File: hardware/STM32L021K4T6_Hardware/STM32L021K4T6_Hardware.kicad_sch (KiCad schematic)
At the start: 1 part, among them U1 STM32L021K4Tx

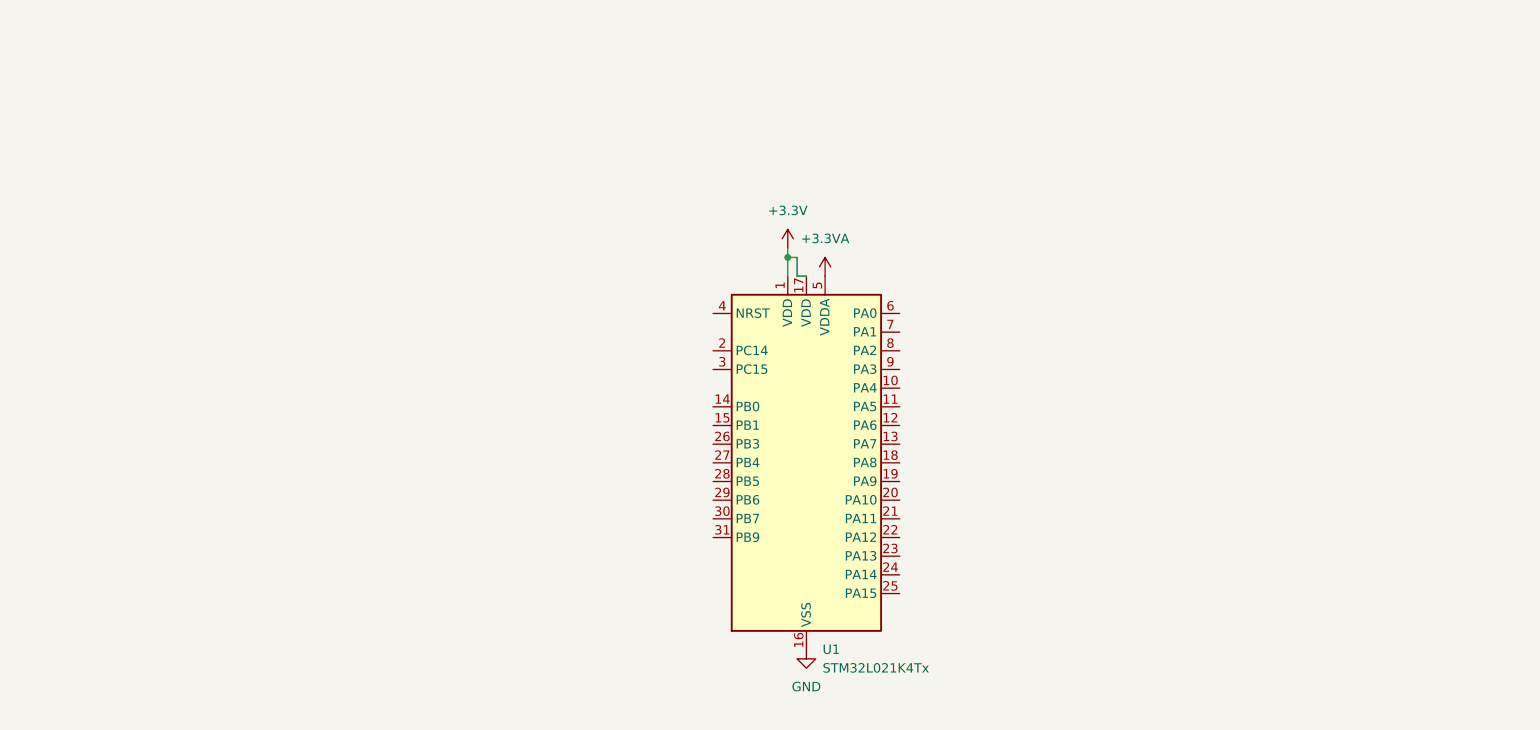
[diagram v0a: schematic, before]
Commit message: schematic and footprints
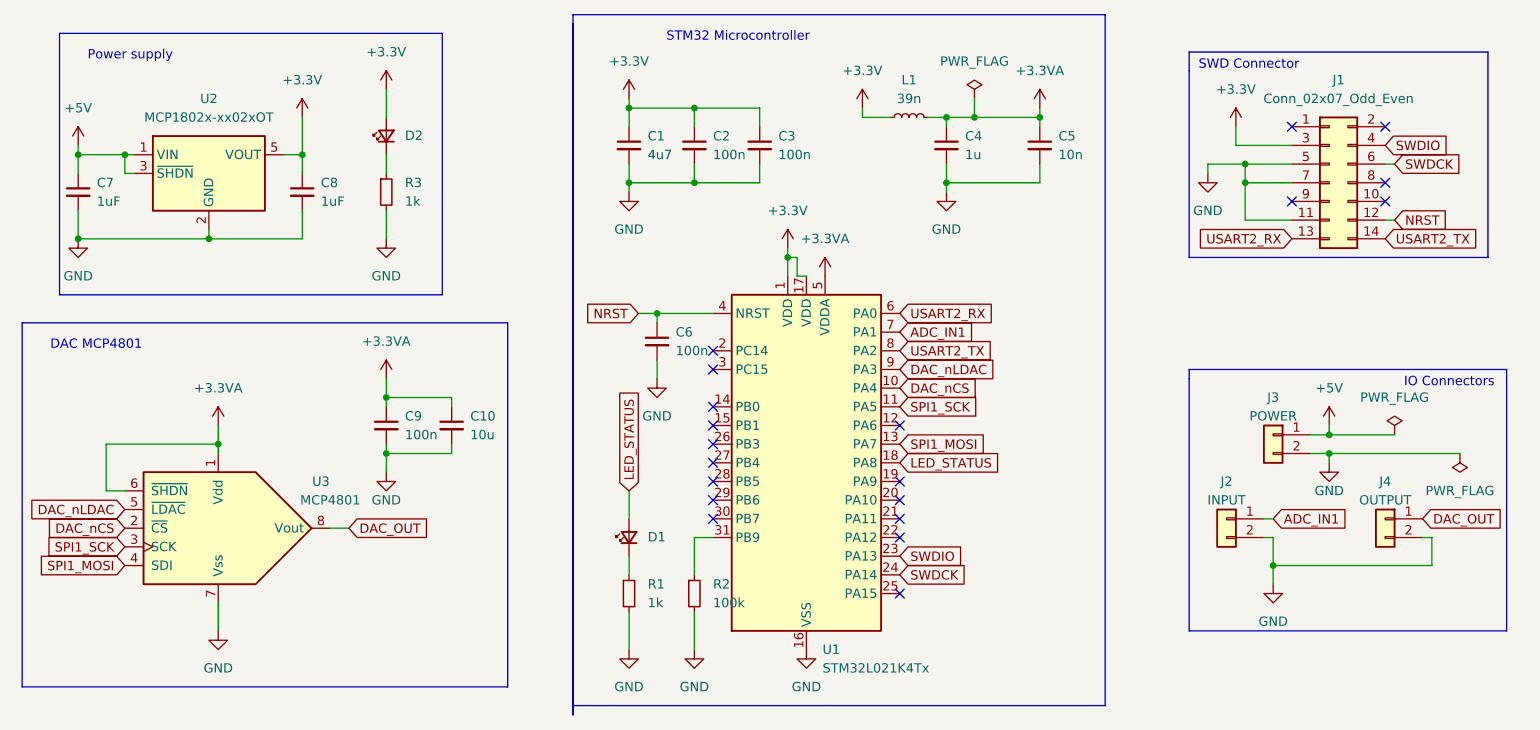
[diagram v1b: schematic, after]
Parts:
- added C1: 4u7, Capacitor_SMD:C_0805_2012Metric_Pad1.18x1.45mm_HandSolder, symbol Device:C_Small
- added C10: 10u, Capacitor_SMD:C_0805_2012Metric, symbol Device:C_Small
- added C2, C3, C6, C9: 100n, Capacitor_SMD:C_0805_2012Metric_Pad1.18x1.45mm_HandSolder, symbol Device:C_Small
- added C4: 1u, Capacitor_SMD:C_0805_2012Metric_Pad1.18x1.45mm_HandSolder, symbol Device:C_Small
- added C5: 10n, Capacitor_SMD:C_0805_2012Metric_Pad1.18x1.45mm_HandSolder, symbol Device:C_Small
- added C7, C8: 1uF, Capacitor_SMD:C_0805_2012Metric, symbol Device:C_Small
- added D1, D2: ~, LED_SMD:LED_0603_1608Metric_Pad1.05x0.95mm_HandSolder, symbol Device:LED_Small
- added J1: Conn_02x07_Odd_Even, Connector_PinHeader_1.27mm:PinHeader_2x07_P1.27mm_Vertical_SMD, symbol Connector_Generic:Conn_02x07_Odd_Even
- added J2: INPUT, Connector_JST:JST_XH_B2B-XH-A_1x02_P2.50mm_Vertical, symbol Connector_Generic:Conn_01x02
- added J3: POWER, Connector_JST:JST_XH_B2B-XH-A_1x02_P2.50mm_Vertical, symbol Connector_Generic:Conn_01x02
- added J4: OUTPUT, Connector_JST:JST_XH_B2B-XH-A_1x02_P2.50mm_Vertical, symbol Connector_Generic:Conn_01x02
- added L1: 39n, Inductor_SMD:L_0805_2012Metric_Pad1.05x1.20mm_HandSolder, symbol Device:L_Small
- added R1, R3: 1k, Resistor_SMD:R_0805_2012Metric_Pad1.20x1.40mm_HandSolder, symbol Device:R_Small
- added R2: 100k, Resistor_SMD:R_0805_2012Metric_Pad1.20x1.40mm_HandSolder, symbol Device:R_Small
- added U2: MCP1802x-xx02xOT, Package_TO_SOT_SMD:SOT-23-5, symbol Regulator_Linear:MCP1802x-xx02xOT
- added U3: MCP4801, Package_SO:SOIC-8_3.9x4.9mm_P1.27mm, symbol Analog_DAC:MCP4801
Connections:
- net +3.3V: now also C1.1, C2.1, C3.1, C8.1, D2.2 (A), J1.3 (Pin_3), L1.1, U2.5 (VOUT)
- net +3.3VA: now also C10.1, C4.1, C5.1, C9.1, L1.2, U3.1 (Vdd), U3.6 (~{SHDN})
- net GND: now also C1.2, C10.2, C2.2, C3.2, C4.2, C5.2, C6.2, C7.2, C8.2, C9.2, J1.11 (Pin_11), J1.5 (Pin_5), J1.7 (Pin_7), J2.2 (Pin_2), J3.2 (Pin_2), J4.2 (Pin_2), R1.2, R2.2, R3.2, U2.2 (GND), U3.7 (Vss)
- net DAC_nCS: now reaches U1.10 (PA4)
- net DAC_nCS: now also U3.2 (~{CS})
- net SPI1_SCK: now reaches U1.11 (PA5)
- net SPI1_SCK: now also U3.3 (SCK)
- net SPI1_MOSI: now reaches U1.13 (PA7)
- net SPI1_MOSI: now also U3.4 (SDI)
- net LED_STATUS: now reaches U1.18 (PA8)
- net LED_STATUS: now also D1.2 (A)
- net SWDIO: now reaches U1.23 (PA13)
- net SWDIO: now also J1.4 (Pin_4)
- net SWDCK: now reaches U1.24 (PA14)
- net SWDCK: now also J1.6 (Pin_6)
- net at U1.31 (PB9): now also R2.1
- net NRST: now reaches U1.4 (NRST)
- net NRST: now also C6.1, J1.12 (Pin_12)
- net USART2_RX: now reaches U1.6 (PA0)
- net USART2_RX: now also J1.13 (Pin_13)
- net ADC_IN1: now reaches U1.7 (PA1)
- net ADC_IN1: now also J2.1 (Pin_1)
- net USART2_TX: now reaches U1.8 (PA2)
- net USART2_TX: now also J1.14 (Pin_14)
- net DAC_nLDAC: now reaches U1.9 (PA3)
- net DAC_nLDAC: now also U3.5 (~{LDAC})
- new net: D1.1 (K), R1.1
- new net: D2.1 (K), R3.1
- new net +5V: C7.1, J3.1 (Pin_1), U2.1 (VIN), U2.3 (~{SHDN})
- new net DAC_OUT: J4.1 (Pin_1), U3.8 (Vout)
- no-connect marks 0 -> 20
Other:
- note added: "DAC MCP4801"
- note added: "IO Connectors"
- note added: "Power supply"
- note added: "STM32 Microcontroller"
- note added: "SWD Connector"
